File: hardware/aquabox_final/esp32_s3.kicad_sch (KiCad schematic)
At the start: 0 parts

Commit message: Atualização
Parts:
- added U2: ESP32-S3-DEVKITC-1-N16R8V, ESP32-S3-DEVKITC-1-N16R8V:XCVR_ESP32-S3-DEVKITC-1-N16R8V, symbol ESP32-S3-DEVKITC-1-N16R8V:ESP32-S3-DEVKITC-1-N16R8V
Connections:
- new net 3V3: U2.J1_1 (3V3), U2.J1_2 (3V3)
- new net GND: U2.J1_22 (GND), U2.J3_1 (GND), U2.J3_21 (GND), U2.J3_22 (GND)

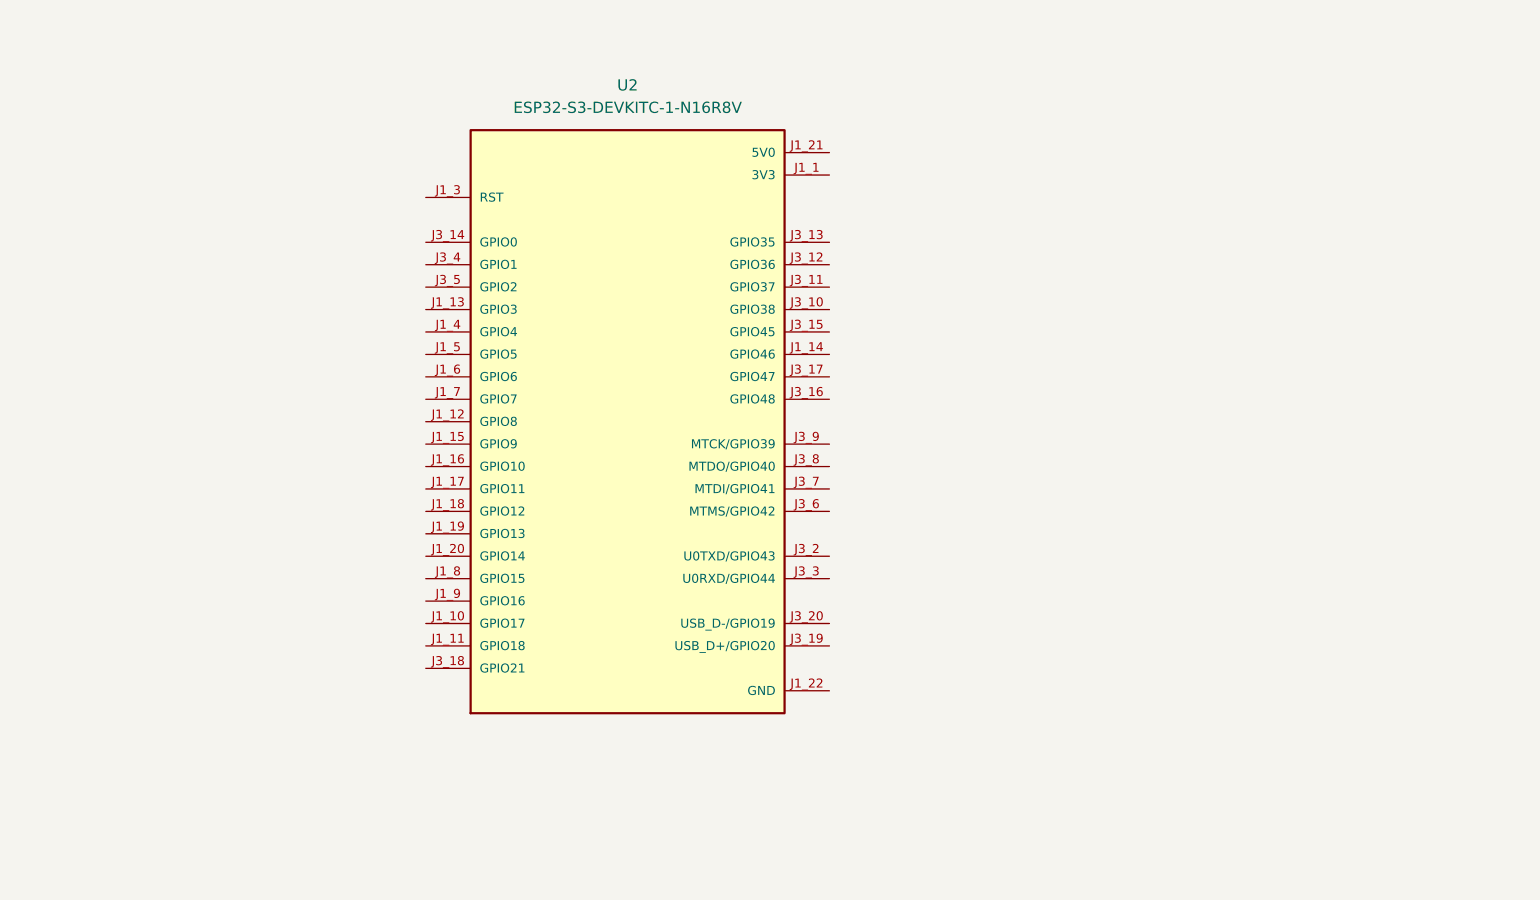
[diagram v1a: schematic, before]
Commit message: Atualização
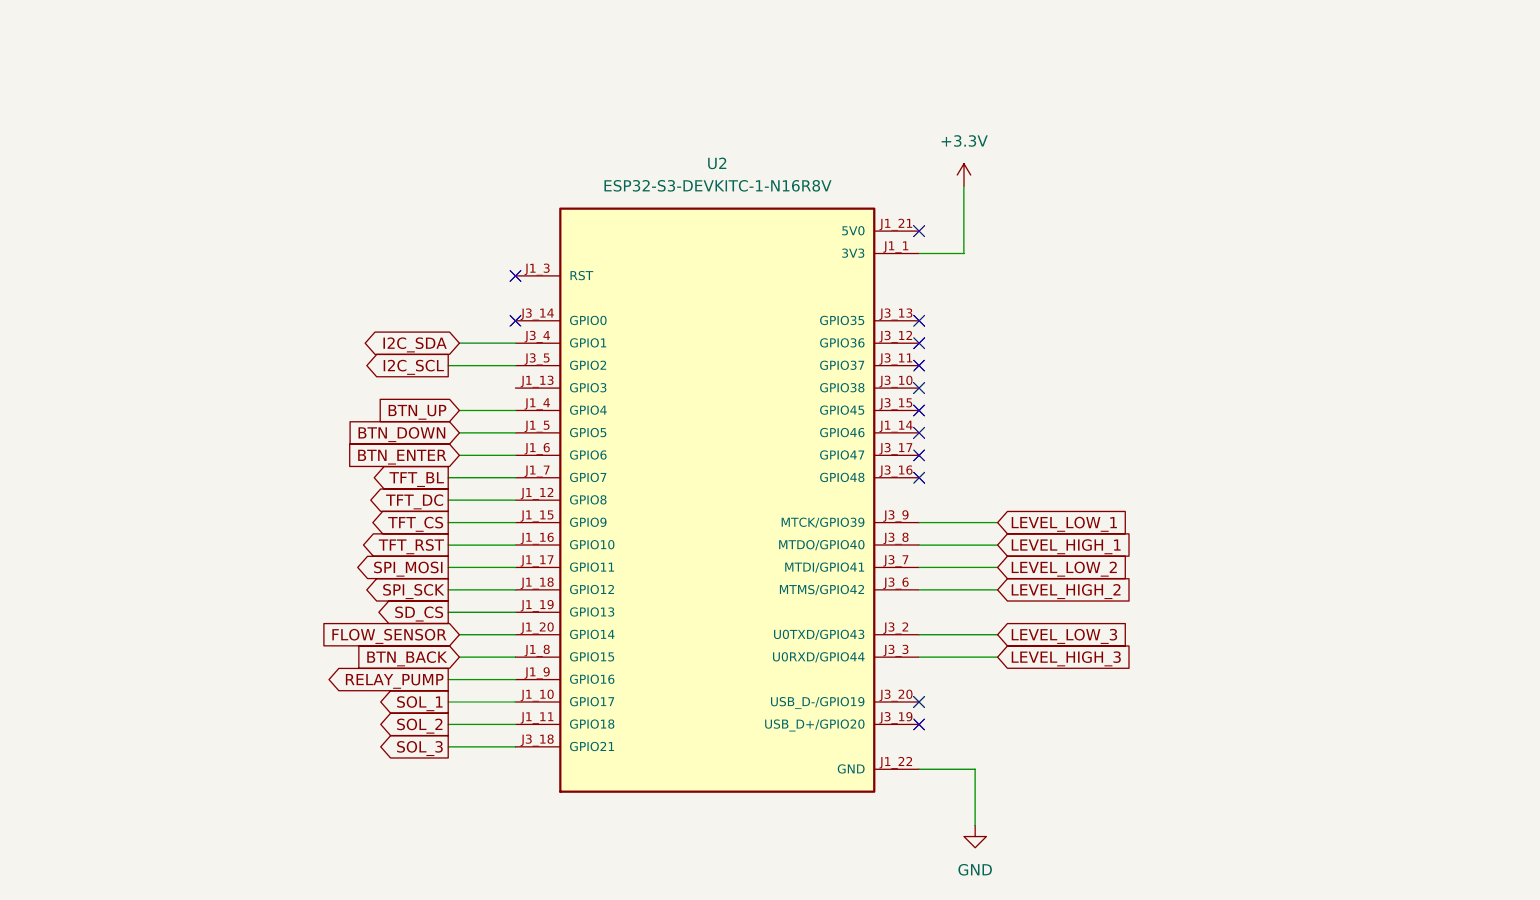
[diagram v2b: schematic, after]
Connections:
- net SOL_1: now reaches U2.J1_10 (GPIO17)
- net SOL_2: now reaches U2.J1_11 (GPIO18)
- net TFT_DC: now reaches U2.J1_12 (GPIO8)
- net TFT_CS: now reaches U2.J1_15 (GPIO9)
- net TFT_RST: now reaches U2.J1_16 (GPIO10)
- net SPI_MOSI: now reaches U2.J1_17 (GPIO11)
- net SPI_SCK: now reaches U2.J1_18 (GPIO12)
- net SD_CS: now reaches U2.J1_19 (GPIO13)
- net FLOW_SENSOR: now reaches U2.J1_20 (GPIO14)
- net BTN_UP: now reaches U2.J1_4 (GPIO4)
- net BTN_DOWN: now reaches U2.J1_5 (GPIO5)
- net BTN_ENTER: now reaches U2.J1_6 (GPIO6)
- net TFT_BL: now reaches U2.J1_7 (GPIO7)
- net BTN_BACK: now reaches U2.J1_8 (GPIO15)
- net RELAY_PUMP: now reaches U2.J1_9 (GPIO16)
- net SOL_3: now reaches U2.J3_18 (GPIO21)
- net LEVEL_LOW_3: now reaches U2.J3_2 (U0TXD/GPIO43)
- net LEVEL_HIGH_3: now reaches U2.J3_3 (U0RXD/GPIO44)
- net I2C_SDA: now reaches U2.J3_4 (GPIO1)
- net I2C_SCL: now reaches U2.J3_5 (GPIO2)
- net LEVEL_HIGH_2: now reaches U2.J3_6 (MTMS/GPIO42)
- net LEVEL_LOW_2: now reaches U2.J3_7 (MTDI/GPIO41)
- net LEVEL_HIGH_1: now reaches U2.J3_8 (MTDO/GPIO40)
- net LEVEL_LOW_1: now reaches U2.J3_9 (MTCK/GPIO39)
- net 3V3 renamed +3.3V
- no-connect marks 0 -> 13
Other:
- moved on the sheet: U2

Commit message: Atualização
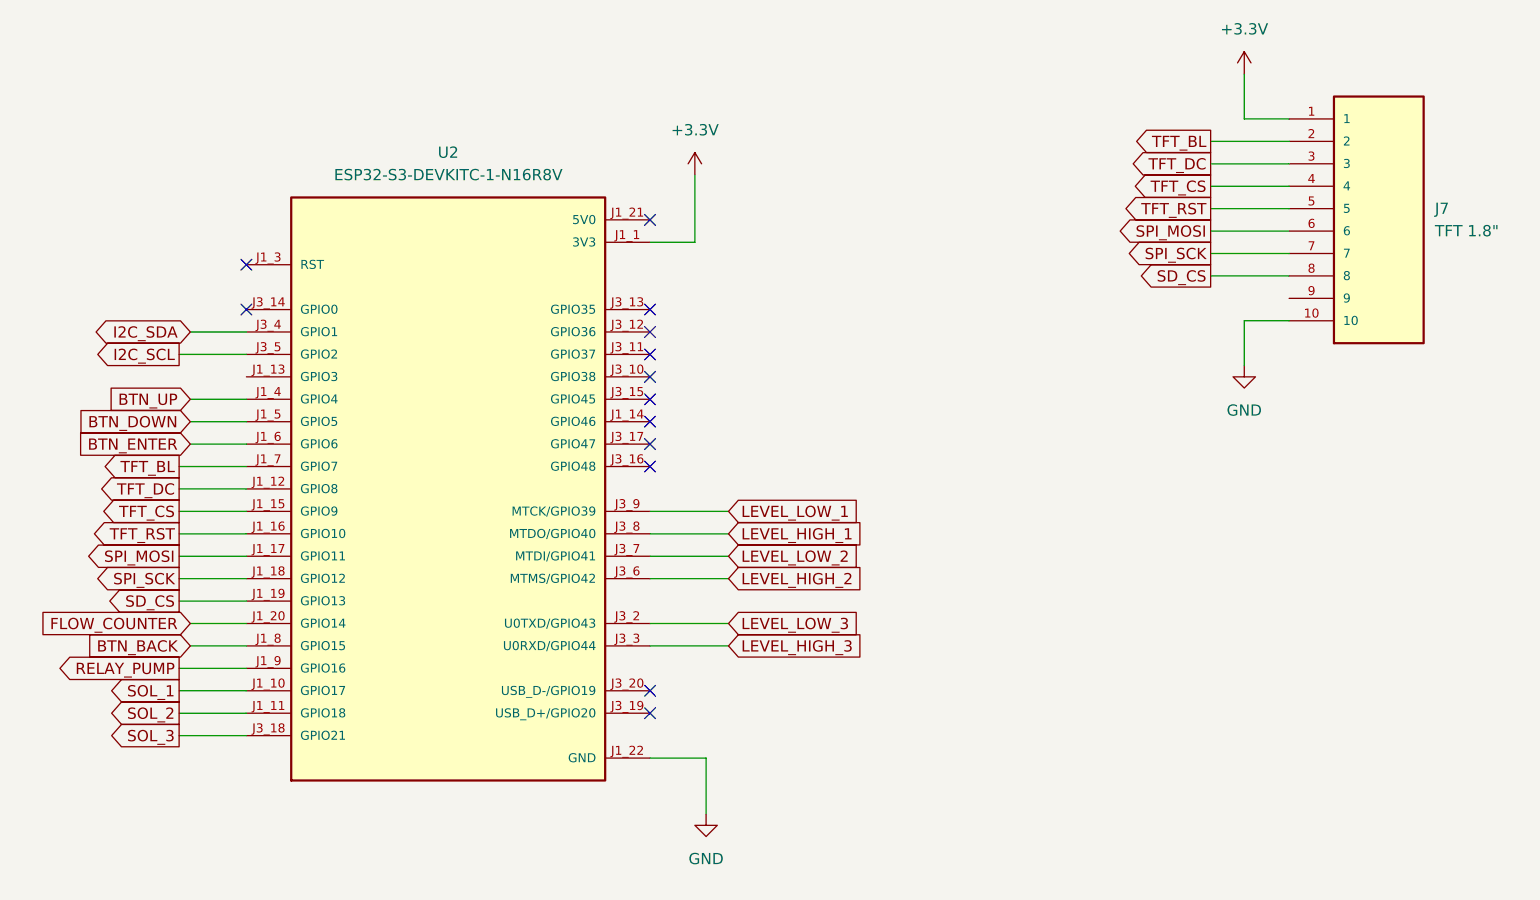
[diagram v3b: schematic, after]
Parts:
- added J7: TFT 1.8{dblquote}, 5104338-1:TE_5104338-1, symbol 5104338-1:5104338-1
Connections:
- net +3.3V: now also J7.1
- net GND: now also J7.10
- net SD_CS: now also J7.8
- net SPI_MOSI: now also J7.6
- net SPI_SCK: now also J7.7
- net TFT_BL: now also J7.2
- net TFT_CS: now also J7.4
- net TFT_DC: now also J7.3
- net TFT_RST: now also J7.5
- net FLOW_SENSOR renamed FLOW_COUNTER
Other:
- company: (none) -> INVENCTUS Soluções Tecnológicas
- title: (none) -> ESP32_S3
- moved on the sheet: U2
